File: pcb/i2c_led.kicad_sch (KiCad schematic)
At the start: 15 parts, among them J1 Conn_01x05, U1 AW9523B

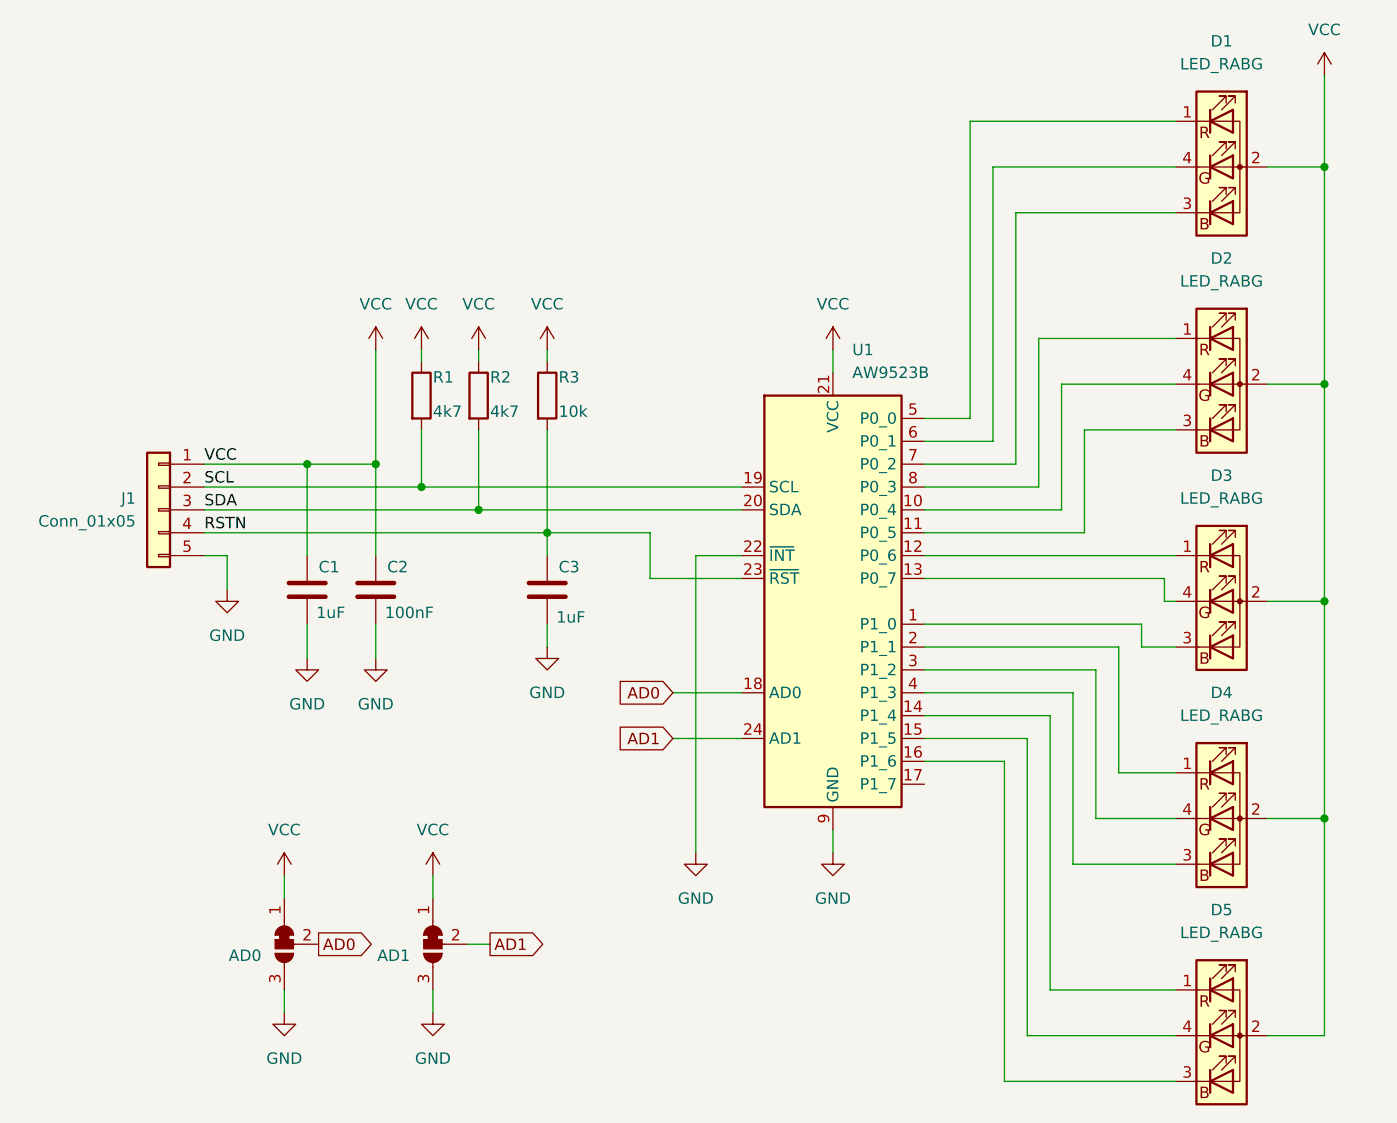
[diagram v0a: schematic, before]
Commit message: More tweaking
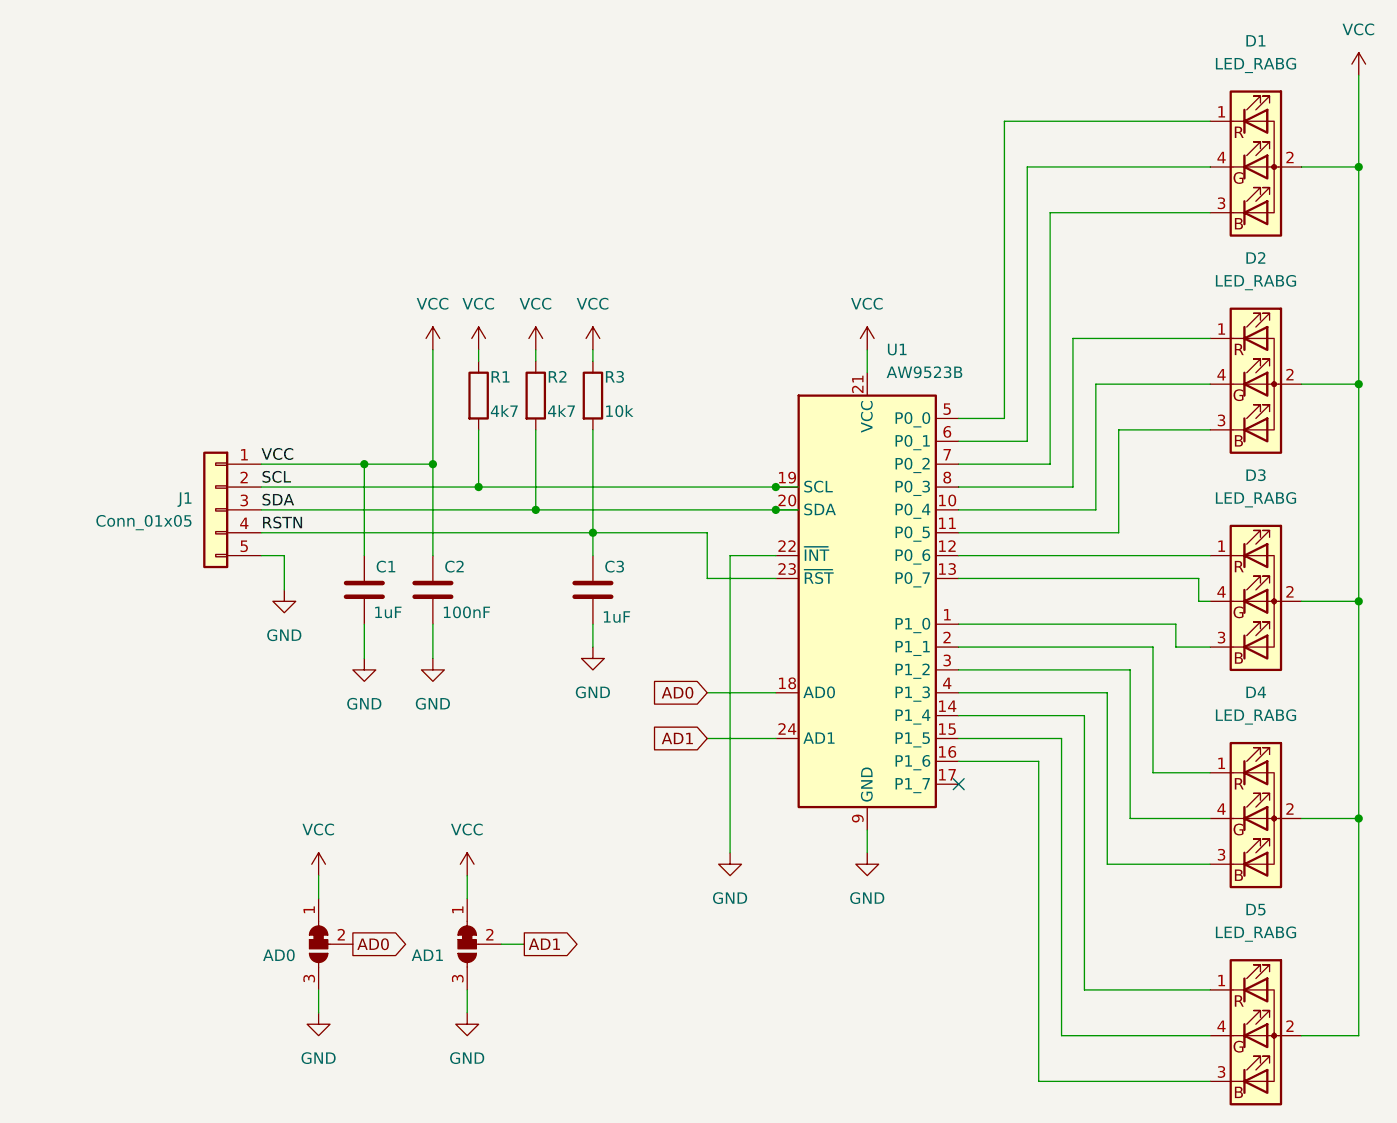
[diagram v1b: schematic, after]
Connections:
- no-connect marks 0 -> 1
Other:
- company: (none) -> ${COMPANY}
- moved on the sheet: AD0, AD1, C1, C2, C3, D1, D2, D3, D4, D5, J1, R1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
